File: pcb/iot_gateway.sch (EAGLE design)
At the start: 184 parts, among them CON1 6P-SH-TOP, CON2 6P-SH-TOP, CON3 2P-PH-TOP, J2 DCJACK-SMD, Q1 AO3401, Q2 AO3401, Q3 AO3400, Q4 AO3400, T1 BC817, T2 BC817, T3 BC817, T4 BC817, T5 BC817, U1 EFM32GG11B4XX_Q100, U10 CCS811, U11 MIC4682, U12 MIC4682, U13 MIC39101, U14 FS312F-G, U15 TP4056, U16 FS8205, U17 ER-TFT035-6, U2 SST26VF064B, U3 SST26VF016B, U4 ESP8266EX, U5 RFM69HW, U6 SIM800C, U7 SI7021, U8 SI7210, U9 BMP280, Y1 8 MHz, Y2 32.768 kHz, Y3 24 MHz

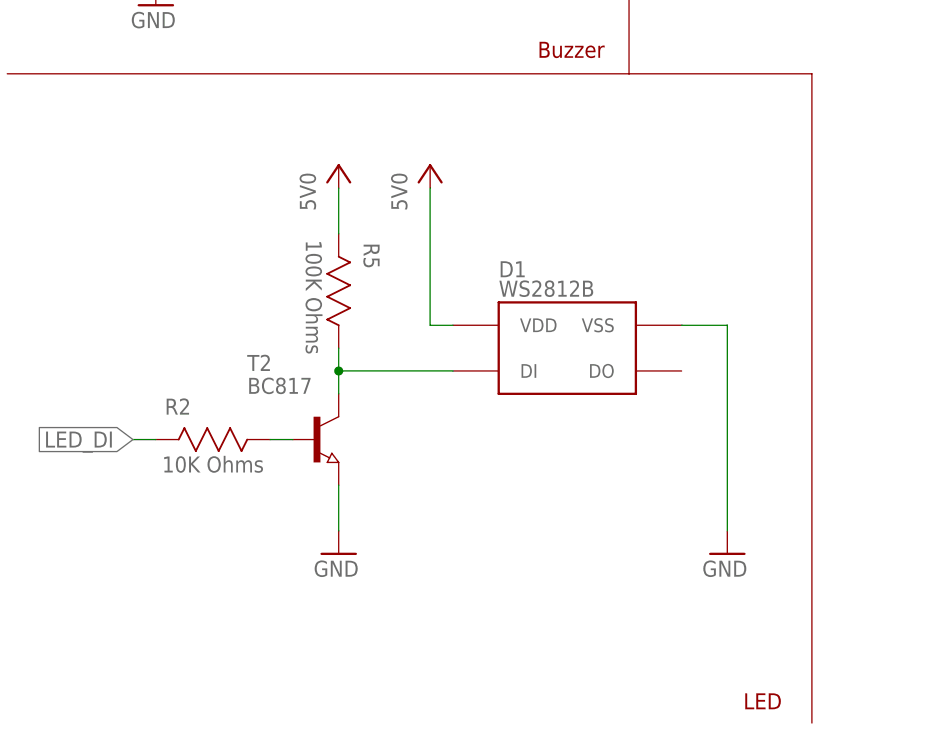
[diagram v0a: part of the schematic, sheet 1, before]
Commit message: Fix hardware errors
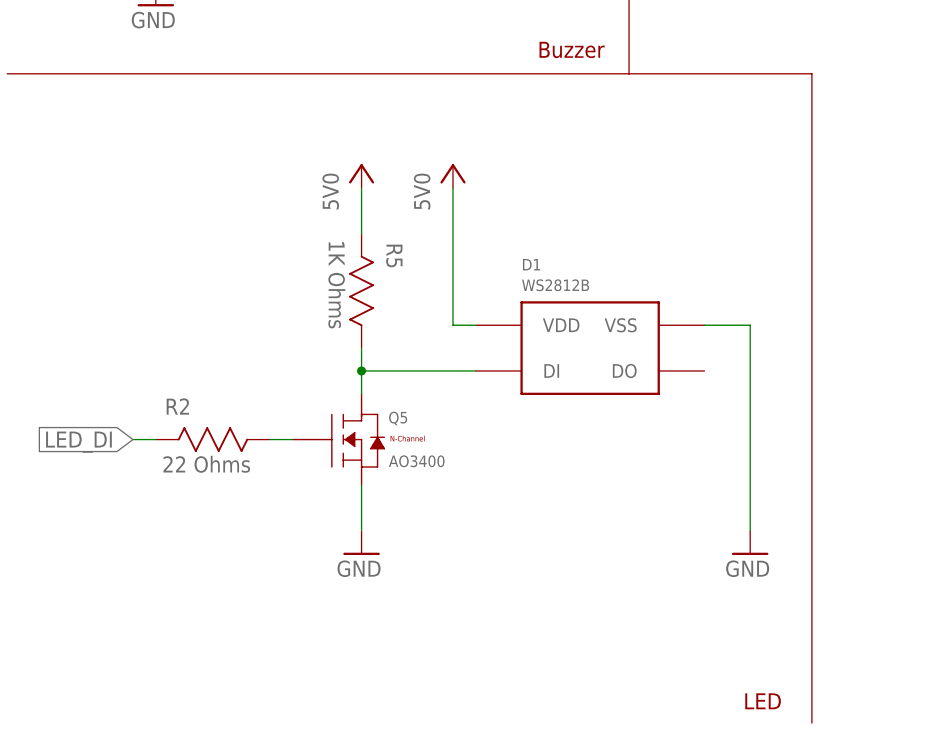
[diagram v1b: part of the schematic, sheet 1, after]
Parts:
- removed T2: BC817, Generic BJT:BC817
- added Q5: AO3400, Alpha Omega:AO3400
- added SJ1: (no value), Solder Jumper:SJS
- R2: value 10K Ohms -> 22 Ohms
- R5: value 100K Ohms -> 1K Ohms
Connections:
- new net N$11: SJ1.1, U4.XPD_DCDC/IO16
- net !WIFI_RST: now also SJ1.2; no longer U4.XPD_DCDC/IO16
- net GND: now also J2.2, Q5.S; no longer J2.3, T2.E
- net N$19: now also Q5.D; no longer T2.C
- net N$32: now also Q5.G; no longer T2.B
- net VIN_DET: now also J2.3; no longer J2.2
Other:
- moved on the sheet: D1, R21, R5
